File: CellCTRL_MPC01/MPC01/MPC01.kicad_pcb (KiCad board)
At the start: 4 copper layers, 95.8 x 62 mm, 51 parts, among them J1 Power 24V, J10 Microstepping, J11 Microstepping, J12 StepMotor 1, J13 StepMotor 2, J14 StepMotor 3, J15 StepMotor 4, J16 Conn_01x05_Pin, J2 Conn_01x03_Pin, J3 Servo Motor 1u2, J4 Endstop X, J5 Endstop Y, J6 Endstop Z, J7 0Ohm Jumper, J8 Microstepping, J9 Microstepping, U1 TP8485E-SR

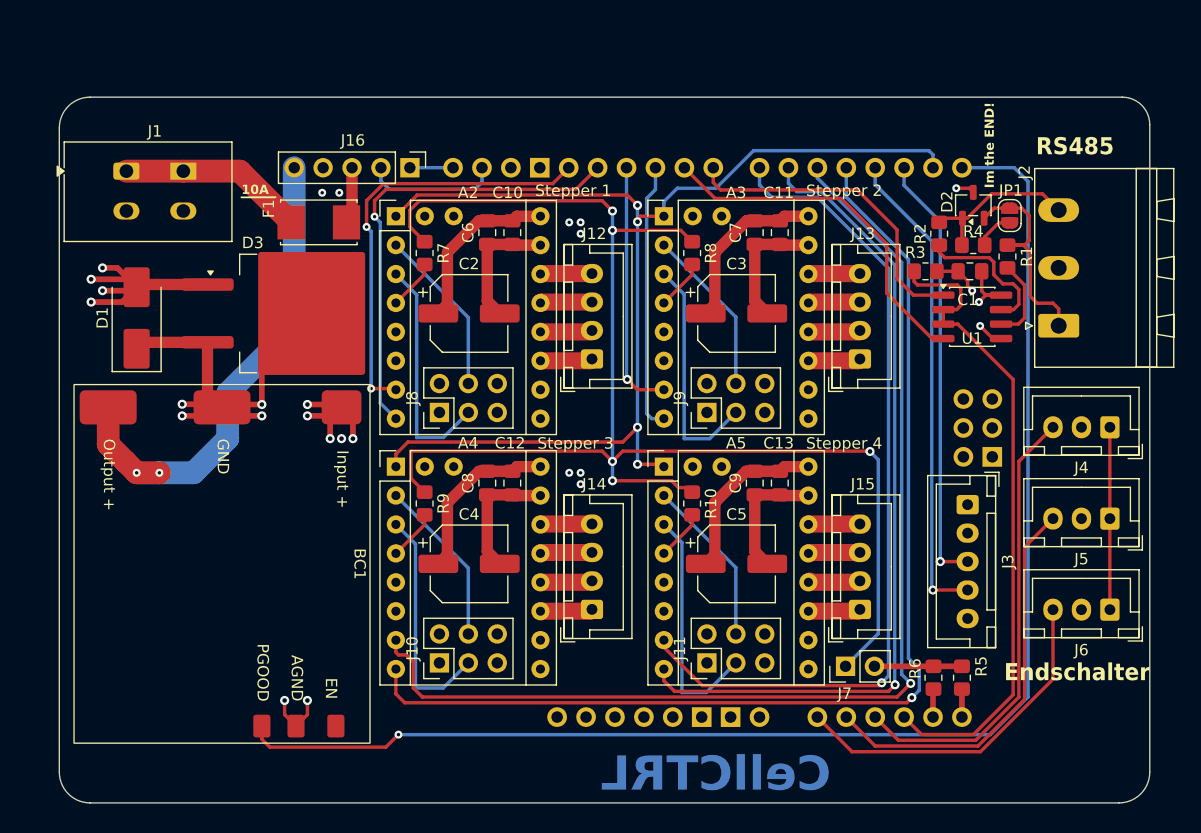
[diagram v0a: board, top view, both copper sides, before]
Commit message: Update MPC01
MPC01 update
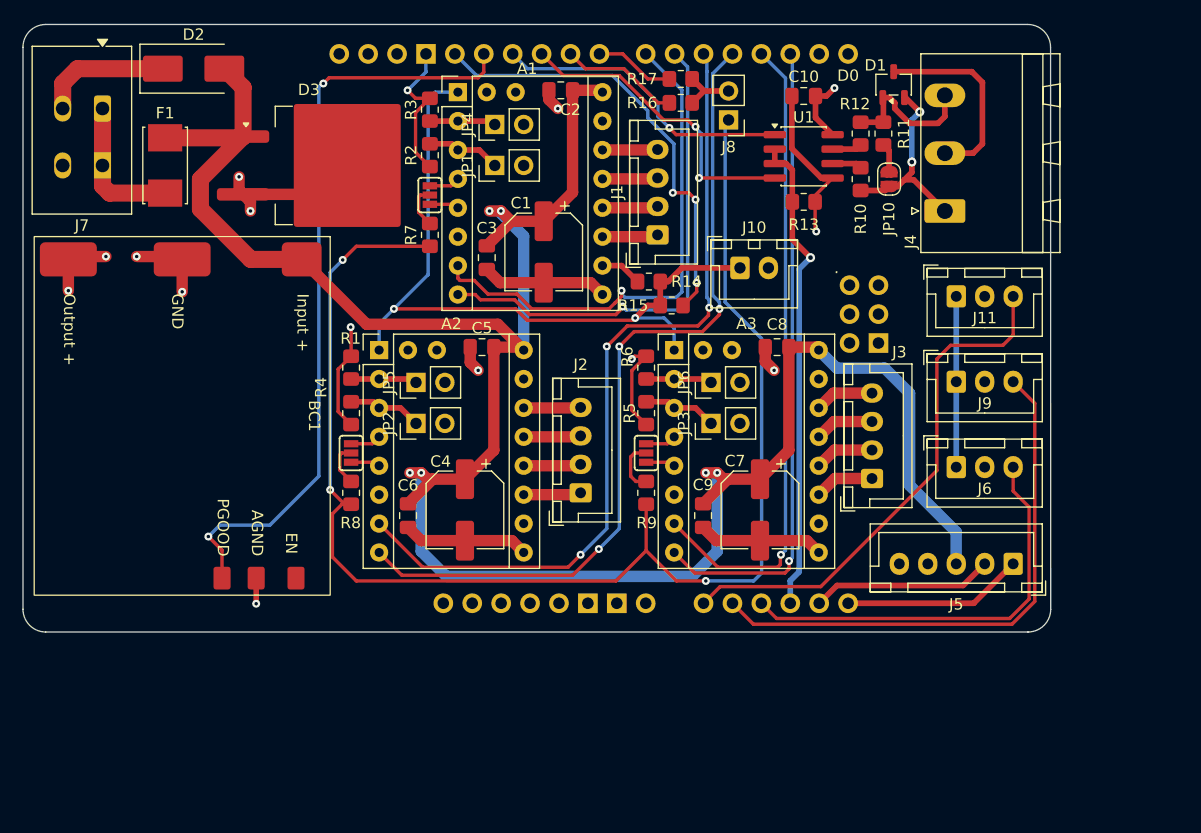
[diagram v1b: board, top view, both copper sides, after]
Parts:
- removed A5: TMC2209, MPC01_lib:TMC2209
- removed C11, C12, C13: 4,7uF, Capacitor_SMD:C_0805_2012Metric_Pad1.18x1.45mm_HandSolder
- removed J12: StepMotor 1, Connector_JST:JST_XH_B4B-XH-A_1x04_P2.50mm_Vertical
- removed J13: StepMotor 2, Connector_JST:JST_XH_B4B-XH-A_1x04_P2.50mm_Vertical
- removed J14: StepMotor 3, Connector_JST:JST_XH_B4B-XH-A_1x04_P2.50mm_Vertical
- removed J15: StepMotor 4, Connector_JST:JST_XH_B4B-XH-A_1x04_P2.50mm_Vertical
- removed J16: Conn_01x05_Pin, Connector_PinHeader_2.54mm:PinHeader_1x05_P2.54mm_Vertical
- added JP10: Jumper_2_Open, Jumper:SolderJumper-2_P1.3mm_Open_RoundedPad1.0x1.5mm, F.Cu at (137.1, 50.2)
- added JP2: MS1, Connector_PinHeader_2.54mm:PinHeader_1x02_P2.54mm_Vertical, F.Cu at (95.5, 71.7)
- added JP3: MS1, Connector_PinHeader_2.54mm:PinHeader_1x02_P2.54mm_Vertical, F.Cu at (121.5, 71.7)
- added JP4: MS2, Connector_PinHeader_2.54mm:PinHeader_1x02_P2.54mm_Vertical, F.Cu at (102.5, 45.4)
- added JP5: MS2, Connector_PinHeader_2.54mm:PinHeader_1x02_P2.54mm_Vertical, F.Cu at (95.5, 68.1)
- added JP6: MS2, Connector_PinHeader_2.54mm:PinHeader_1x02_P2.54mm_Vertical, F.Cu at (121.5, 68.1)
- added JP7: Jumper_3_Open, PCM_SparkFun-Jumper:Jumper_3_NO, F.Cu at (96.8, 51.6)
- added JP8: Jumper_3_Open, PCM_SparkFun-Jumper:Jumper_3_NO, F.Cu at (89.8, 74.3)
- added JP9: Jumper_3_Open, PCM_SparkFun-Jumper:Jumper_3_NO, F.Cu at (115.8, 74.3)
- added R11: 120R, Resistor_SMD:R_0805_2012Metric_Pad1.20x1.40mm_HandSolder, F.Cu at (136.6, 46.2)
- added R12: 10R, Resistor_SMD:R_0805_2012Metric_Pad1.20x1.40mm_HandSolder, F.Cu at (134.6, 46.2)
- added R13: 10K, Resistor_SMD:R_0805_2012Metric_Pad1.20x1.40mm_HandSolder, F.Cu at (129.6, 52.2)
- added R14: 10K, Resistor_SMD:R_0805_2012Metric_Pad1.20x1.40mm_HandSolder, F.Cu at (116.0, 59.2)
- added R15: 1K, Resistor_SMD:R_0805_2012Metric_Pad1.20x1.40mm_HandSolder, F.Cu at (118.0, 61.3)
- added R16: 1K, Resistor_SMD:R_0805_2012Metric_Pad1.20x1.40mm_HandSolder, F.Cu at (118.8, 43.5)
- added R17: 1K, Resistor_SMD:R_0805_2012Metric_Pad1.20x1.40mm_HandSolder, F.Cu at (118.8, 41.4)
- A1: value Arduino_Uno_R3_Shield -> TMC2209; footprint PCM_arduino-library:Arduino_Uno_R3_Shield -> MPC01_lib:TMC2209
- A4: value TMC2209 -> Arduino_Uno_R3_Shield; footprint MPC01_lib:TMC2209 -> PCM_arduino-library:Arduino_Uno_R3_Shield
- C1: value 100n -> 100uf; footprint Capacitor_SMD:C_0805_2012Metric_Pad1.18x1.45mm_HandSolder -> Capacitor_SMD:CP_Elec_6.3x7.7
- C10: value 4,7uF -> 100n
- C2, C5: value 100uf -> 1uF; footprint Capacitor_SMD:CP_Elec_6.3x7.7 -> Capacitor_SMD:C_0805_2012Metric_Pad1.18x1.45mm_HandSolder
- C3: value 100uf -> 4,7uF; footprint Capacitor_SMD:CP_Elec_6.3x7.7 -> Capacitor_SMD:C_0805_2012Metric_Pad1.18x1.45mm_HandSolder
- C6, C9: value 1uF -> 4,7uF
- C7: value 1uF -> 100uf; footprint Capacitor_SMD:C_0805_2012Metric_Pad1.18x1.45mm_HandSolder -> Capacitor_SMD:CP_Elec_6.3x7.7
- D1: value D_TVS -> SM712_SOT23; footprint Diode_SMD:D_SMB_Handsoldering -> Package_TO_SOT_SMD:SOT-23-3
- D2: value SM712_SOT23 -> D_TVS; footprint Package_TO_SOT_SMD:SOT-23-3 -> Diode_SMD:D_SMB_Handsoldering
- J1: value Power 24V -> StepMotor 1; footprint TerminalBlock_WAGO:TerminalBlock_WAGO_2601-1102_1x02_P3.50mm_Horizontal -> Connector_JST:JST_XH_B4B-XH-A_1x04_P2.50mm_Vertical
- J10: value Microstepping -> Enable/Disable; footprint MPC01_lib:PinHeader_2x03_P2.54mm_Vertical_ Pinorder -> Connector_JST:JST_XH_B2B-XH-A_1x02_P2.50mm_Vertical
- J11: value Microstepping -> Endstop Z; footprint MPC01_lib:PinHeader_2x03_P2.54mm_Vertical_ Pinorder -> Connector_JST:JST_XH_B3B-XH-A_1x03_P2.50mm_Vertical
- J2: value Conn_01x03_Pin -> StepMotor 2; footprint Connector_Phoenix_MSTB:PhoenixContact_MSTBA_2,5_3-G-5,08_1x03_P5.08mm_Horizontal -> Connector_JST:JST_XH_B4B-XH-A_1x04_P2.50mm_Vertical
- J3: value Servo Motor 1u2 -> StepMotor 3; footprint Connector_JST:JST_XH_B5B-XH-A_1x05_P2.50mm_Vertical -> Connector_JST:JST_XH_B4B-XH-A_1x04_P2.50mm_Vertical
- J4: value Endstop X -> Conn_01x03_Pin; footprint Connector_JST:JST_XH_B3B-XH-A_1x03_P2.50mm_Vertical -> Connector_Phoenix_MSTB:PhoenixContact_MSTBA_2,5_3-G-5,08_1x03_P5.08mm_Horizontal
- J5: value Endstop Y -> I2C; footprint Connector_JST:JST_XH_B3B-XH-A_1x03_P2.50mm_Vertical -> Connector_JST:JST_XH_B5B-XH-A_1x05_P2.50mm_Vertical
- J6: value Endstop Z -> Endstop X
- J7: value 0Ohm Jumper -> Power 24V; footprint Connector_PinHeader_2.54mm:PinHeader_1x02_P2.54mm_Vertical -> TerminalBlock_WAGO:TerminalBlock_WAGO_2601-1102_1x02_P3.50mm_Horizontal
- J8: value Microstepping -> 0Ohm Jumper; footprint MPC01_lib:PinHeader_2x03_P2.54mm_Vertical_ Pinorder -> Connector_PinHeader_2.54mm:PinHeader_1x02_P2.54mm_Vertical
- J9: value Microstepping -> Endstop Y; footprint MPC01_lib:PinHeader_2x03_P2.54mm_Vertical_ Pinorder -> Connector_JST:JST_XH_B3B-XH-A_1x03_P2.50mm_Vertical
- JP1: value Jumper_2_Open -> MS1; footprint Jumper:SolderJumper-2_P1.3mm_Open_RoundedPad1.0x1.5mm -> Connector_PinHeader_2.54mm:PinHeader_1x02_P2.54mm_Vertical
- R1, R2: value 10R -> 10K
- R10: value 1K -> 10R
- R4: value 120R -> 10K
- R5, R6: value 1K -> 10K
- moved J7 81.6 mm to (68.0, 44.0), turned to 180 degrees
- moved D1 69.6 mm to (137.5, 41.9)
- moved D2 69.5 mm to (76.0, 40.5), turned to 0 degrees
- moved A1 61.5 mm to (97.8, 41.1)
- moved R1 58.5 mm to (89.8, 66.8), turned to -90 degrees
- moved R4 56.6 mm to (89.8, 70.8), turned to 90 degrees
- moved J1 47.0 mm to (116.8, 55.1), turned to 90 degrees
- moved R3 45.8 mm to (96.8, 44.1), turned to -90 degrees
- moved JP1 45.5 mm to (102.5, 49.0)
- moved R2 45.3 mm to (96.8, 48.1)
- moved J2 44.5 mm to (110.0, 77.8)
- moved J10 43.6 mm to (124.0, 58.0), turned to 0 degrees
- moved J11 38.9 mm to (143.0, 60.5), turned to 0 degrees
- moved C1 37.5 mm to (106.8, 56.6), turned to -90 degrees
- moved R6 37.1 mm to (115.8, 66.8), turned to -90 degrees
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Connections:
- A2 pad 5: unconnected-(A2-TX-Pad5) -> Net-(A2-TX)
- A2 pad 7: STEP1 -> STEP2
- A2 pad 8: DIR1 -> DIR2
- A3 pad 5: unconnected-(A3-TX-Pad5) -> Net-(A3-TX)
- A3 pad 7: STEP2 -> STEP3
- A3 pad 8: DIR2 -> DIR3
- C1 pad 1: 5V -> +24V
- C10 pad 1: GND -> 5V
- C10 pad 2: +24V -> GND
- C2 pad 1: +24V -> GND
- C2 pad 2: GND -> +24V
- C3 pad 1: +24V -> GND
- C3 pad 2: GND -> +24V
- C5 pad 1: +24V -> GND
- C5 pad 2: GND -> +24V
- C7 pad 1: GND -> +24V
- C7 pad 2: +24V -> GND
- D1 pad 1: GND -> Net-(D1-A1)
- D1 pad 2: +24V -> Net-(D1-A2)
- D2 pad 1: Net-(D2-A1) -> GND
- D2 pad 2: Net-(D2-A2) -> +24V
- F1 pad 2: Net-(J1-Pin_1) -> Net-(J7-Pin_1)
- J1 pad 1: Net-(J1-Pin_1) -> Net-(A1-B2)
- J1 pad 2: GND -> Net-(A1-B1)
- J10 pad 1: 5V -> ENABLE
- J10 pad 2: Net-(A4-MS2) -> GND
- J11 pad 1: 5V -> Net-(J11-Pin_1)
- J11 pad 2: Net-(A5-MS2) -> GND
- J11 pad 3: GND -> EndstopZ
- J2 pad 1: Net-(D2-A2) -> Net-(A2-B2)
- J2 pad 2: GND -> Net-(A2-B1)
- J2 pad 3: Net-(D2-A1) -> Net-(A2-A1)
- J3 pad 1: GND -> Net-(A3-B2)
- J3 pad 2: 5V -> Net-(A3-B1)
- J3 pad 3: Motor1 -> Net-(A3-A1)
- J3 pad 4: Motor2 -> Net-(A3-A2)
- J4 pad 1: Net-(J4-Pin_1) -> Net-(D1-A2)
- J4 pad 3: EndstopX -> Net-(D1-A1)
- J5 pad 1: Net-(J4-Pin_1) -> Net-(J5-Pin_1)
- J5 pad 2: GND -> Net-(J5-Pin_2)
- J5 pad 3: EndstopY -> +24V
- J6 pad 1: Net-(J4-Pin_1) -> Net-(J11-Pin_1)
- J6 pad 3: EndstopZ -> EndstopX
- J7 pad 1: PDNUart -> Net-(J7-Pin_1)
- J7 pad 2: Net-(J7-Pin_2) -> GND
- J8 pad 1: 5V -> PDNUart
- J8 pad 2: Net-(A2-MS2) -> Net-(J8-Pin_2)
- J9 pad 1: 5V -> Net-(J11-Pin_1)
- J9 pad 2: Net-(A3-MS2) -> GND
- J9 pad 3: GND -> EndstopY
- JP1 pad 1: Net-(JP1-A) -> Net-(A1-MS2)
- JP1 pad 2: Net-(D2-A2) -> 5V
- R1 pad 1: RS485_A -> GND
- R1 pad 2: Net-(D2-A2) -> Net-(A2-MS1)
- R10 pad 1: PDNUart -> RS485_A
- R10 pad 2: Net-(A5-RX) -> Net-(D1-A2)
- R2 pad 1: RS485_B -> GND
- R2 pad 2: Net-(D2-A1) -> Net-(A1-MS2)
- R3 pad 1: RS485_DE/RE -> GND
- R3 pad 2: GND -> Net-(A1-MS1)
- R4 pad 1: Net-(JP1-A) -> GND
- R4 pad 2: Net-(D2-A1) -> Net-(A2-MS2)
- R5 pad 1: RX -> GND
- R5 pad 2: Net-(J7-Pin_2) -> Net-(A3-MS2)
- R6 pad 1: TX -> GND
- R6 pad 2: Net-(J7-Pin_2) -> Net-(A3-MS1)
- R7 pad 1: PDNUart -> Net-(JP7-C)
- R7 pad 2: Net-(A2-RX) -> PDNUart
- R8 pad 1: PDNUart -> Net-(JP8-C)
- R8 pad 2: Net-(A3-RX) -> PDNUart
- R9 pad 1: PDNUart -> Net-(JP9-C)
- R9 pad 2: Net-(A4-RX) -> PDNUart
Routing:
- net STEP4: track 73.8 -> 0.00 mm, vias 1 -> 0
- net DIR4: track 72.5 -> 0.00 mm, vias 1 -> 0
- net PGOOD: track 122.2 -> 66.9 mm, vias 1 -> 2
- net STEP2: track 22.2 -> 72.4 mm, vias 1 -> 3
- net DIR2: track 23.6 -> 73.5 mm, vias 0 -> 3
- net Motor2: track 42.3 -> 0.00 mm, vias 1 -> 0
- net STEP3: track 98.5 -> 56.9 mm
- net DIR3: track 97.5 -> 56.4 mm
- net ENABLEOut: track 0.00 -> 39.3 mm, vias 0 -> 3
- net GND: track 99.2 -> 137.6 mm, vias 9 -> 12
- net Motor1: track 38.3 -> 0.00 mm, vias 1 -> 0
- net ENABLE: track 101.6 -> 66.4 mm, vias 4 -> 2
- net 5V: track 50.0 -> 15.8 mm
- net Net-(A5-MS2): track 21.2 -> 0.00 mm
- net Net-(A4-MS2): track 20.6 -> 0.00 mm
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- removed copper zone on In2.Cu, net +24V
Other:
- board size 95.8 x 62 mm -> 90.3 x 53.4 mm
- board text added: "(I2C)"
- board text added: "24V"
- board text added: "5V"
- board text added: "GND"
- board text added: "Motor 1 (X)"
- board text added: "Motor 2 (Y)"
- board text added: "Motor 3 (Z)"
- board text added: "Power In (24V DC)"
- board text added: "SCL"
- board text added: "SDA"
- board text added: "X-Endstop"
- board text added: "Y-Endstop"
- board text added: "Z-Endstop"
- board text removed: "10A"
- board text removed: "2026/02 V0.1b Edited by: KJ"
- board text removed: "CellCTRL"
- board text removed: "Endschalter"
- board text removed: "Im the END!"
- board text removed: "MPC01"
- board text removed: "Stepper 1"
- board text removed: "Stepper 2"
- board text removed: "Stepper 3"
- board text removed: "Stepper 4"
- board text removed: "This Product is designed and made for KTLA/Litec"
